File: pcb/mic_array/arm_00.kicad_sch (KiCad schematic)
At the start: 16 parts, among them U1 IM72D128V01XTMA1, U2 IM72D128V01XTMA1, U3 IM72D128V01XTMA1, U4 IM72D128V01XTMA1, U5 IM72D128V01XTMA1, U6 IM72D128V01XTMA1, U7 IM72D128V01XTMA1, U8 IM72D128V01XTMA1

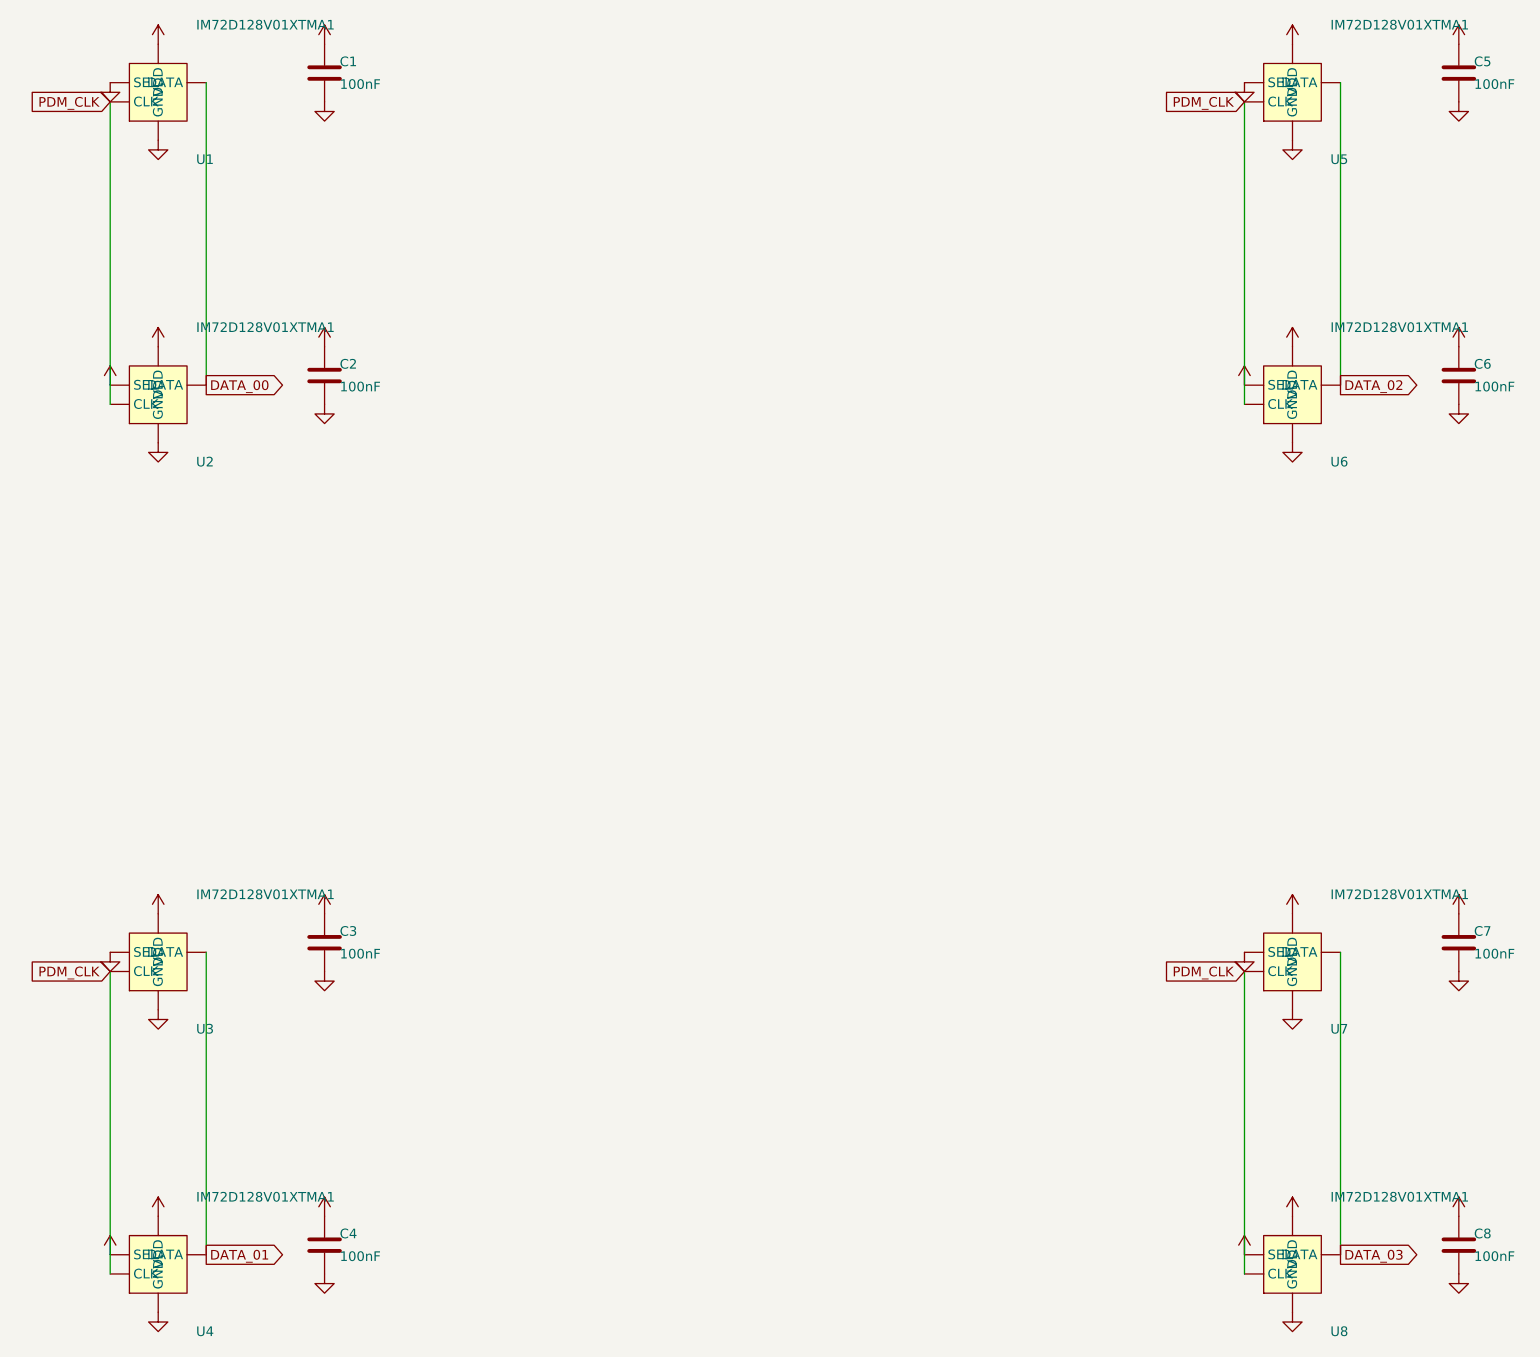
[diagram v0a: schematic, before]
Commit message: Updated.
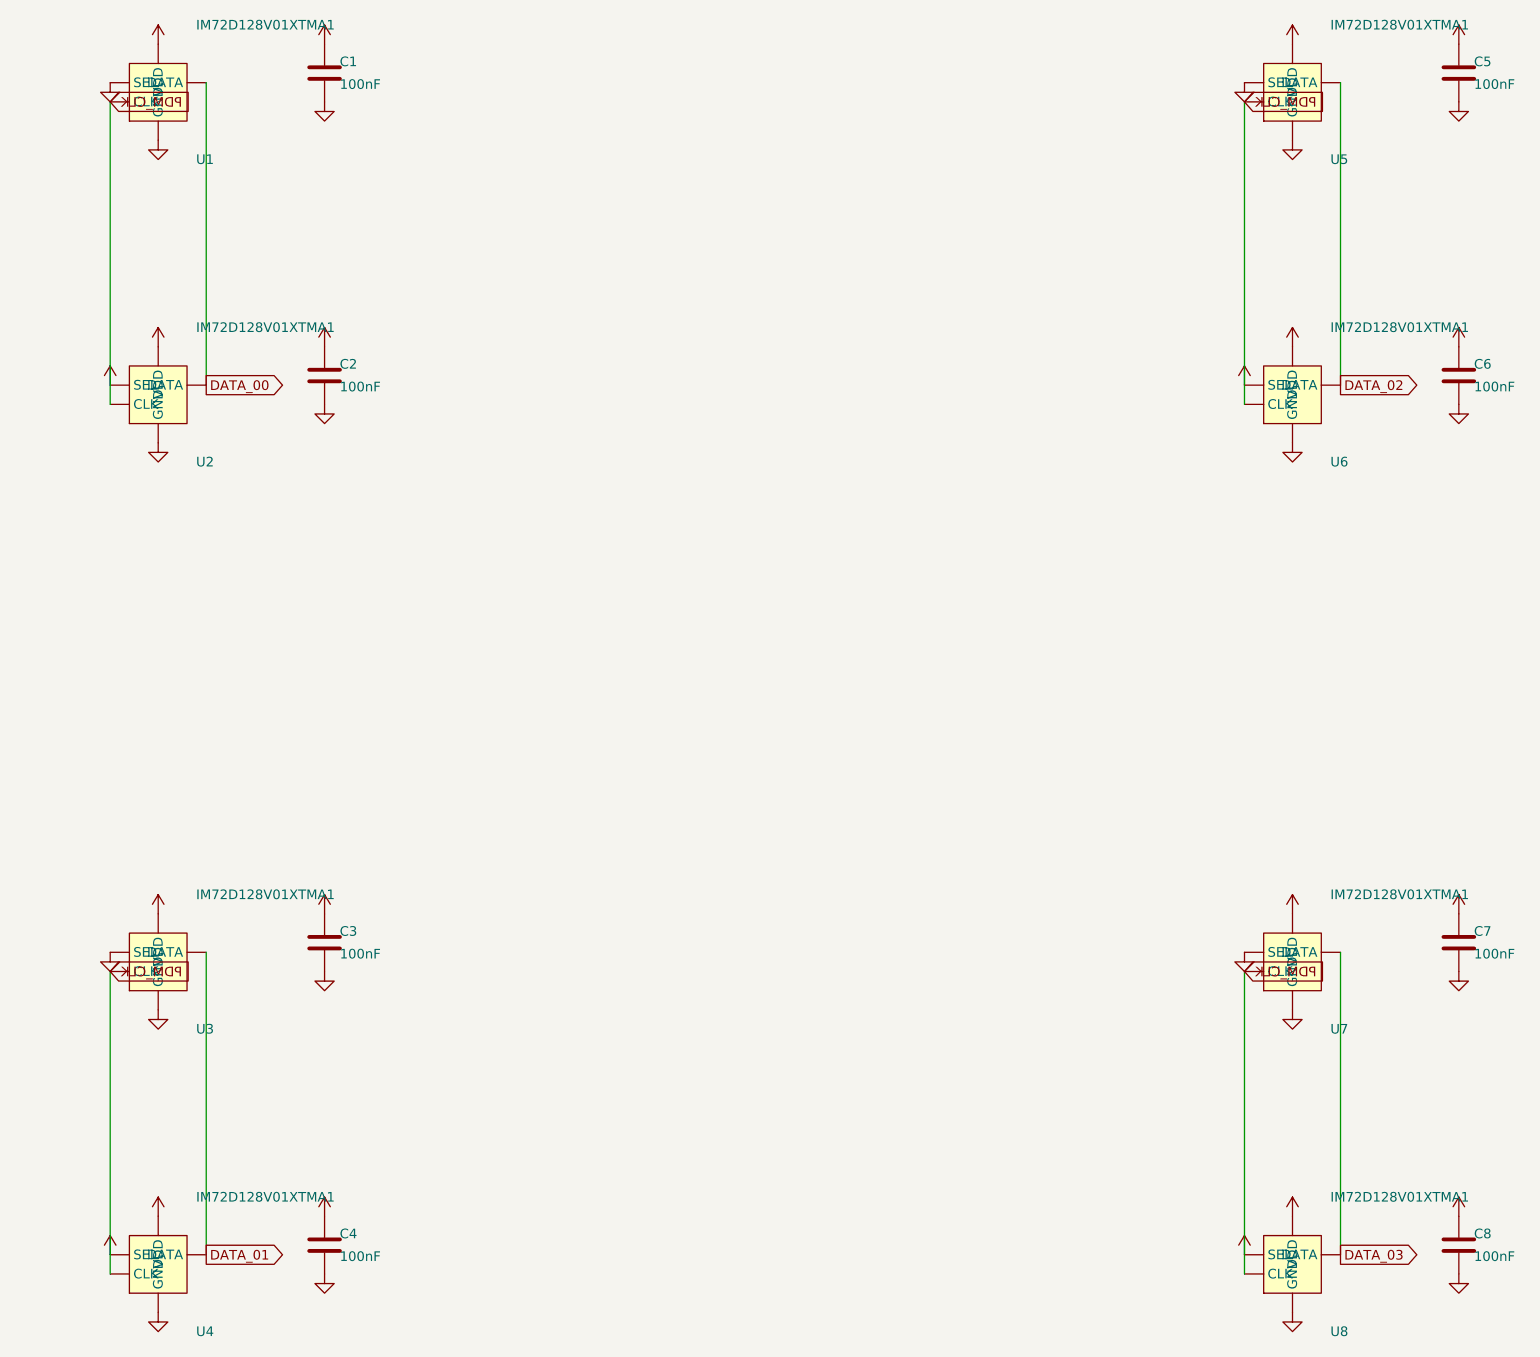
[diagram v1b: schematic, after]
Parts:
- C1, C2, C3, C4, C5, C6, C7, C8: footprint Capacitor_SMD:C_0402_1005Metric -> (none)
- U1, U2, U3, U4, U5, U6, U7, U8: footprint Sensor_Audio:Infineon_PG-LLGA-5-2 -> (none)
